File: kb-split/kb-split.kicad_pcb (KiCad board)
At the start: 2 copper layers, 166.2 x 88.1 mm, 125 parts, among them J1 USB_C_Receptacle_USB2.0, J2 Conn_01x03_Male, SW1 SW_PUSH, SW10 SW_PUSH, SW11 SW_PUSH, SW12 SW_PUSH, SW13 SW_PUSH, SW14 SW_PUSH, SW15 Rotary_Encoder_Switch, SW16 SW_PUSH, SW17 SW_PUSH, SW18 SW_PUSH, SW19 SW_PUSH, SW2 SW_PUSH, SW20 SW_PUSH, SW21 SW_PUSH, SW22 SW_PUSH, SW23 SW_PUSH, SW24 SW_PUSH, SW25 SW_PUSH, SW26 SW_PUSH, SW27 SW_PUSH, SW28 SW_PUSH, SW3 SW_PUSH, SW4 SW_PUSH, SW5 SW_PUSH, SW6 SW_PUSH, SW7 SW_PUSH, SW8 SW_PUSH, SW9 SW_PUSH, U1 SRV05-4, U2 ATmega32U4-AU, Y1 Crystal_GND24_Small

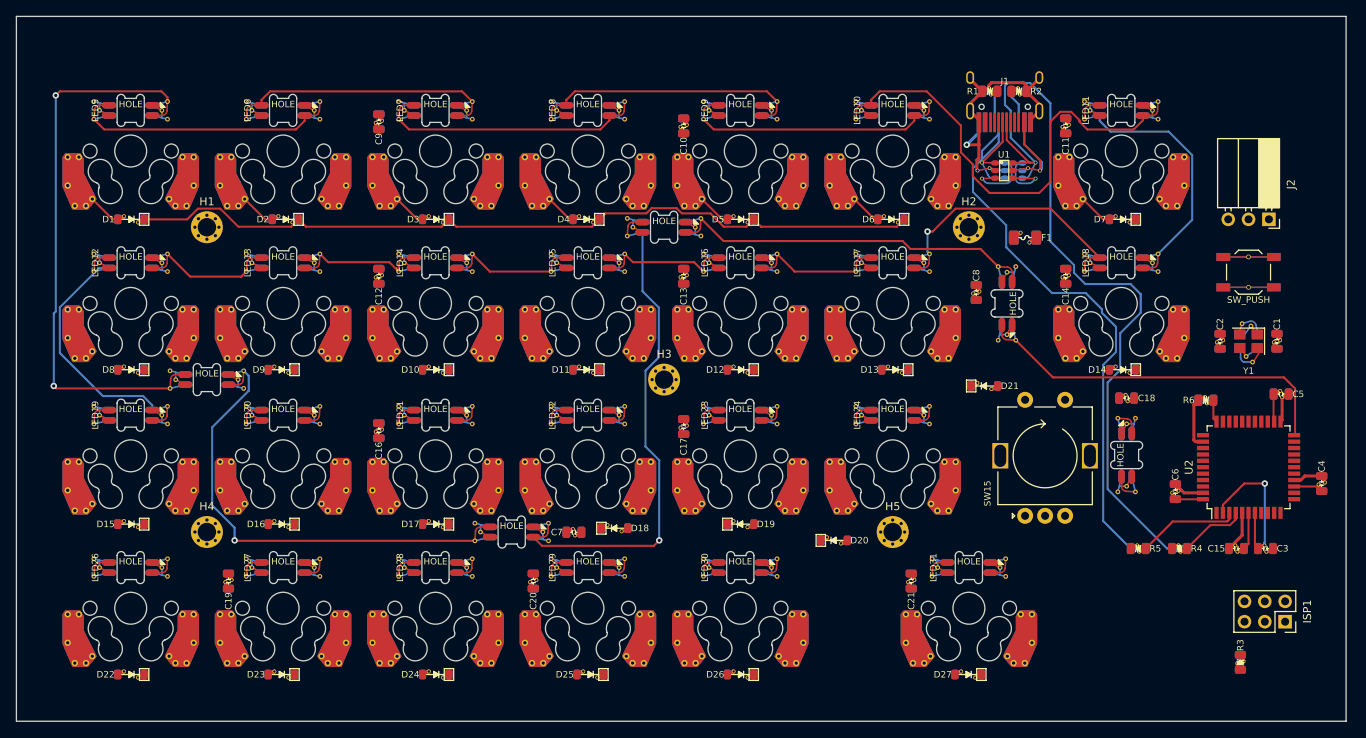
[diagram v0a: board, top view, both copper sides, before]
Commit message: Done routing.
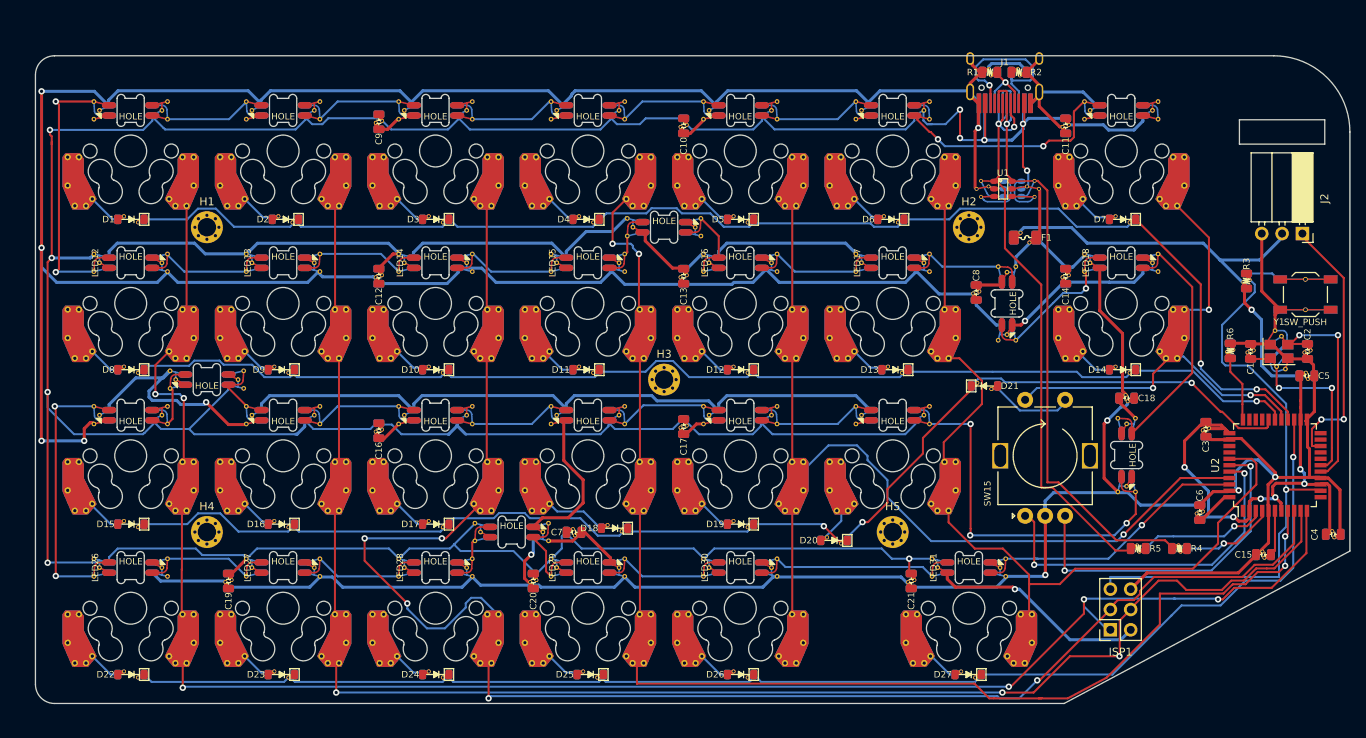
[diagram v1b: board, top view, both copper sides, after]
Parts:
- LED10, LED11, LED19, LED20, LED21, LED22, LED23, LED24, LED5, LED6, LED7, LED8, LED9: moved to B.Cu
- moved R3 47.7 mm to (246.6, 75.8)
- moved ISP1 21.9 mm to (229.6, 119.4), turned to 180 degrees
- moved C3 16.7 mm to (241.6, 94.3), turned to 270 degrees
- moved C2 11.0 mm to (254.3, 84.6)
- moved SW22 7.64 mm to (254.0, 77.5)
- moved R6 6.89 mm to (244.6, 84.5), turned to 90 degrees
- moved C4 6.51 mm to (257.5, 107.4), turned to 0 degrees
- moved J2 4.55 mm to (253.6, 69.8)
- moved C6 4.02 mm to (240.8, 104.7)
- moved Y1 4.02 mm to (250.7, 84.6), turned to 0 degrees
- moved C5 3.95 mm to (254.2, 87.6)
- moved C1 3.54 mm to (247.1, 84.6), turned to 270 degrees
- moved C15 3.47 mm to (248.7, 110.0)
- moved U2 3.31 mm to (250.2, 98.8)
- moved J1 2.38 mm to (216.4, 45.4)
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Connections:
- C7 pad 1: VBUS -> GND
- C7 pad 2: GND -> VBUS
- C8 pad 1: VBUS -> GND
- C8 pad 2: GND -> VBUS
- ISP1 pad 1: MISO -> COL0
- ISP1 pad 2: Net-(ISP1-Pad2) -> VBUS
- ISP1 pad 3: SCK -> COL2
- ISP1 pad 4: MOSI -> COL1
- J2 pad 2: VBUS -> +5V
- LED16 pad 2: Net-(LED15-Pad4) -> Net-(LED16-Pad2)
- LED18 pad 2: Net-(LED17-Pad4) -> Net-(LED18-Pad2)
- LED18 pad 4: Net-(LED11-Pad2) -> Net-(LED18-Pad4)
- LED19 pad 2: Net-(LED19-Pad2) -> Net-(LED1-Pad4)
- LED19 pad 4: Net-(LED12-Pad2) -> Net-(LED19-Pad4)
- LED2 pad 2: Net-(LED1-Pad4) -> Net-(LED2-Pad2)
- LED20 pad 4: Net-(LED19-Pad2) -> Net-(LED1-Pad2)
- LED25 pad 2: Net-(LED25-Pad2) -> Net-(LED18-Pad4)
- LED26 pad 2: Net-(LED26-Pad2) -> Net-(LED19-Pad4)
- LED28 pad 4: Net-(LED28-Pad4) -> Net-(LED2-Pad2)
- LED29 pad 2: Net-(LED28-Pad4) -> Net-(LED2-Pad4)
- LED3 pad 2: Net-(LED2-Pad4) -> Net-(LED15-Pad4)
- LED3 pad 3: GND -> Net-(LED3-Pad3)
- LED3 pad 4: Net-(LED3-Pad4) -> Net-(LED16-Pad2)
- LED31 pad 4: Net-(LED25-Pad2) -> LED
- LED4 pad 1: GND -> VBUS
- LED4 pad 2: Net-(LED3-Pad4) -> Net-(LED17-Pad4)
- LED4 pad 3: VBUS -> GND
- LED4 pad 4: LED -> Net-(LED18-Pad2)
- LED5 pad 4: Net-(LED1-Pad2) -> Net-(LED12-Pad2)
- SW13 pad 1: Net-(SW13-Pad1) -> COL5
- SW14 pad 1: Net-(SW14-Pad1) -> COL6
- SW15 pad S2: Net-(SW14-Pad1) -> COL6
- SW21 pad 1: Net-(SW13-Pad1) -> COL5
- SW28 pad 1: Net-(SW13-Pad1) -> COL5
- SW6 pad 1: Net-(SW13-Pad1) -> COL5
- SW7 pad 1: Net-(SW14-Pad1) -> COL6
- U2 pad 10: MOSI -> COL1
- U2 pad 11: MISO -> COL0
- U2 pad 18: ENC0 -> Net-(U2-Pad18)
- U2 pad 19: ENC1 -> Net-(U2-Pad19)
- U2 pad 22: LED -> Net-(U2-Pad22)
- U2 pad 26: ROW2 -> ROW0
- U2 pad 27: ROW1 -> COL6
- U2 pad 28: ROW0 -> ROW1
- U2 pad 29: COL6 -> ROW2
- U2 pad 30: COL5 -> Net-(U2-Pad30)
- U2 pad 31: COL4 -> Net-(U2-Pad31)
- U2 pad 32: COL3 -> Net-(U2-Pad32)
- U2 pad 36: COL2 -> Net-(U2-Pad36)
- U2 pad 37: COL1 -> Net-(U2-Pad37)
- U2 pad 38: COL0 -> COL5
- U2 pad 39: Net-(U2-Pad39) -> ENC1
- U2 pad 40: Net-(U2-Pad40) -> ENC0
- U2 pad 41: Net-(U2-Pad41) -> COL4
- U2 pad 42: Net-(U2-Pad42) -> LED
- U2 pad 8: Net-(U2-Pad8) -> COL3
- U2 pad 9: SCK -> COL2
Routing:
- net GND: track 54.2 -> 807.5 mm, vias 1 -> 12
- net VBUS: track 13.9 -> 665.5 mm, vias 0 -> 11
- net COL0: track 0.00 -> 208.8 mm, vias 0 -> 6
- net COL2: track 0.00 -> 199.7 mm, vias 0 -> 5
- net COL1: track 0.00 -> 184.8 mm, vias 0 -> 3
- net ROW3: track 0.00 -> 170.5 mm, vias 0 -> 1
- net ROW2: track 0.00 -> 159.6 mm, vias 0 -> 3
- net COL3: track 0.00 -> 151.1 mm, vias 0 -> 4
- net ROW1: track 0.00 -> 149.7 mm, vias 0 -> 1
- net COL4: track 0.00 -> 123.8 mm, vias 0 -> 1
- net +5V: track 30.3 -> 125.2 mm, vias 1 -> 7
- net COL5: track 0.00 -> 92.9 mm
- net RESET: track 0.00 -> 76.4 mm, vias 0 -> 1
- net ROW0: track 101.1 -> 166.9 mm, vias 0 -> 2
- net Net-(LED1-Pad2): track 66.1 -> 3.64 mm, vias 2 -> 0
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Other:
- board size 166.2 x 88.1 mm -> 164.3 x 81 mm
